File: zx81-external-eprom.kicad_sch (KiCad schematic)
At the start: 10 parts, among them J1 Connector ZX81, Q1 BC549, SW1 SW_DIP_x03, U1 W27C512, U2 74LS138

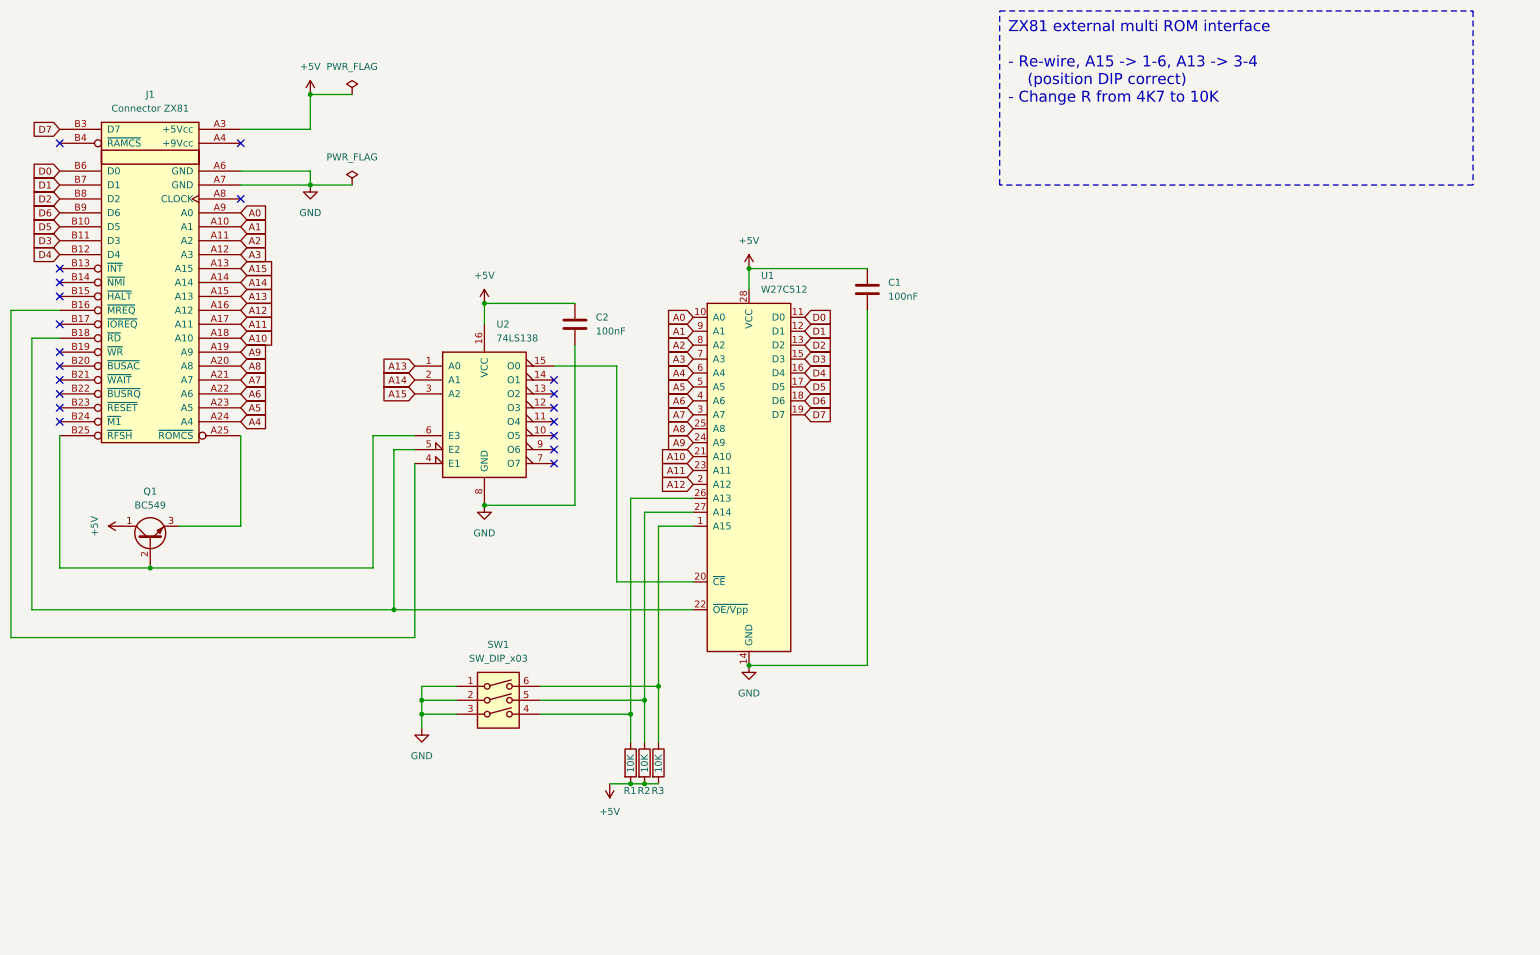
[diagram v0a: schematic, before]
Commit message: version 1.2
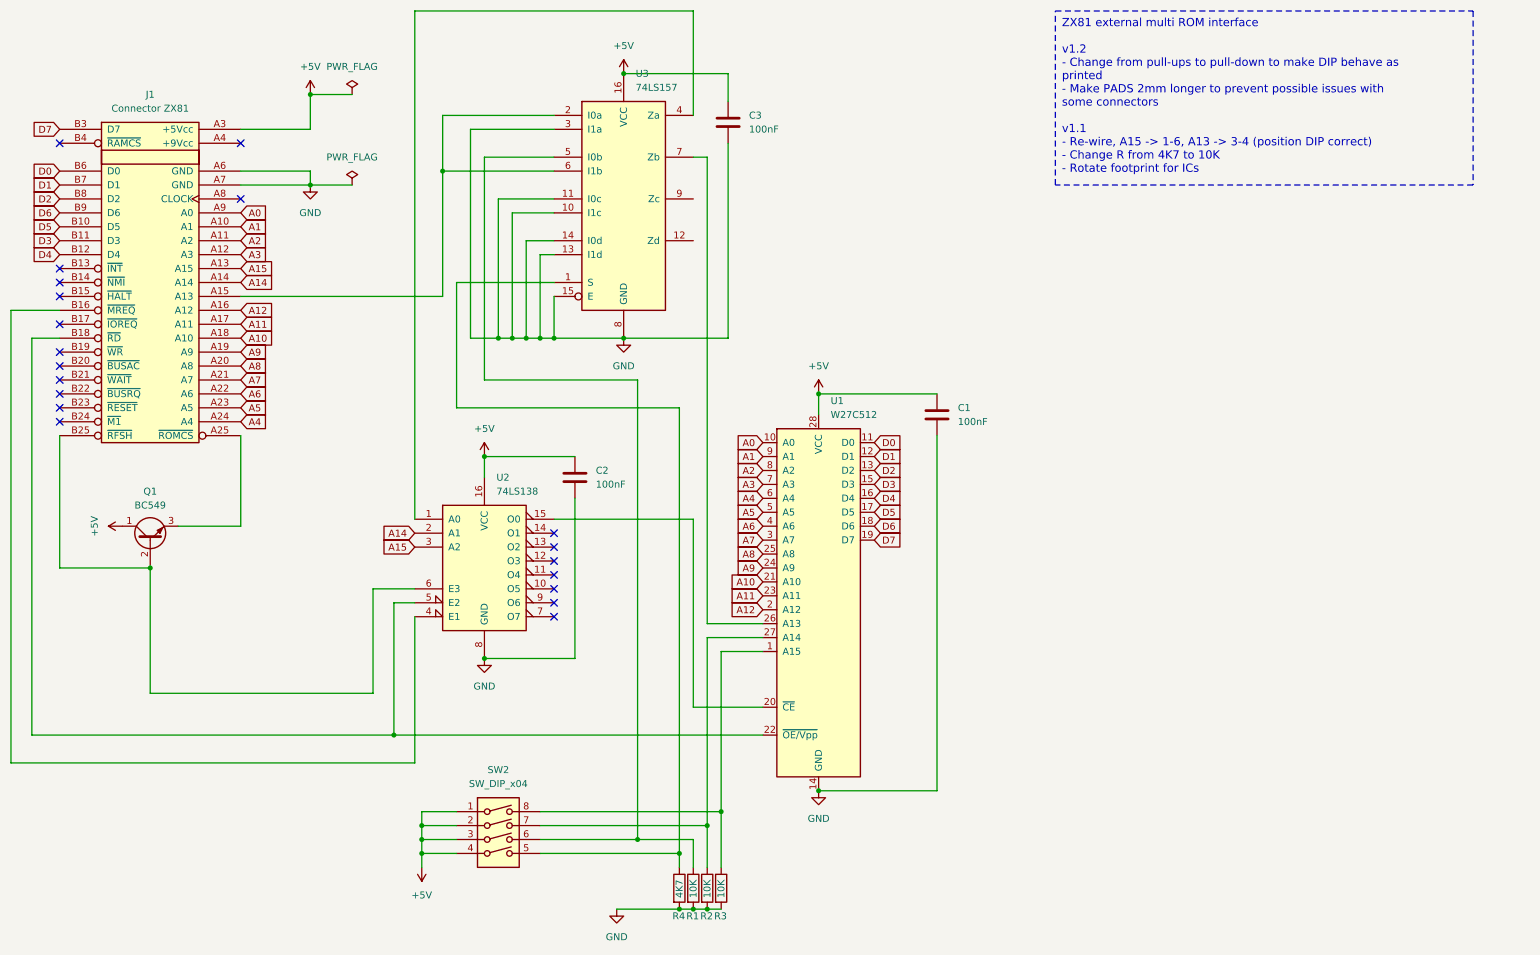
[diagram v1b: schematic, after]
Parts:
- removed SW1: SW_DIP_x03, Button_Switch_THT:SW_DIP_SPSTx03_Slide_6.7x9.18mm_W7.62mm_P2.54mm_LowProfile, symbol Switch:SW_DIP_x03
- added C3: 100nF, Capacitor_THT:C_Disc_D3.0mm_W1.6mm_P2.50mm, symbol Device:C
- added R4: 4K7, Resistor_THT:R_Axial_DIN0207_L6.3mm_D2.5mm_P10.16mm_Horizontal, symbol Device:R
- added SW2: SW_DIP_x04, Button_Switch_THT:SW_DIP_SPSTx04_Slide_6.7x11.72mm_W7.62mm_P2.54mm_LowProfile, symbol Switch:SW_DIP_x04
- added U3: 74LS157, Package_DIP:DIP-16_W7.62mm, symbol 74xx:74LS157
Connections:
- net +5V: now also C3.1, SW2.1, SW2.2, SW2.3, SW2.4, U3.16 (VCC); no longer R1.2, R2.2, R3.2
- net GND: now also R1.2, R2.2, R3.2, C3.2, R4.2, U3.10 (I1c), U3.11 (I0c), U3.13 (I1d), U3.14 (I0d), U3.15 (E), U3.3 (I1a), U3.8 (GND)
- net at R3.1, U1.1 (A15): now also SW2.8
- net at U1.26 (A13): now also U3.7 (Zb); no longer R1.1
- net at R2.1, U1.27 (A14): now also SW2.7
- net A13: no longer names the net of U2.1 (A0)
- net A13: now also U3.4 (Za); no longer J1.A15 (A13)
- new net: R4.1, SW2.5, U3.1 (S)
- new net: R1.1, SW2.6, U3.5 (I0b)
- new net: J1.A15 (A13), U3.2 (I0a), U3.6 (I1b)
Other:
- moved on the sheet: C1, C2, R1, R2, R3, U1, U2
